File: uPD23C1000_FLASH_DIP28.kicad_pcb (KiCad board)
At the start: 2 copper layers, 16.6 x 34.4 mm, 8 parts, among them J1 uPD23C1000, J2 Conn_1x2, J3 Conn_1x3, U1 29F010 TSOP-32 20mm, U2 29F010 sTSOP-32 14mm, U3 29F010 PLCC-32 7x9

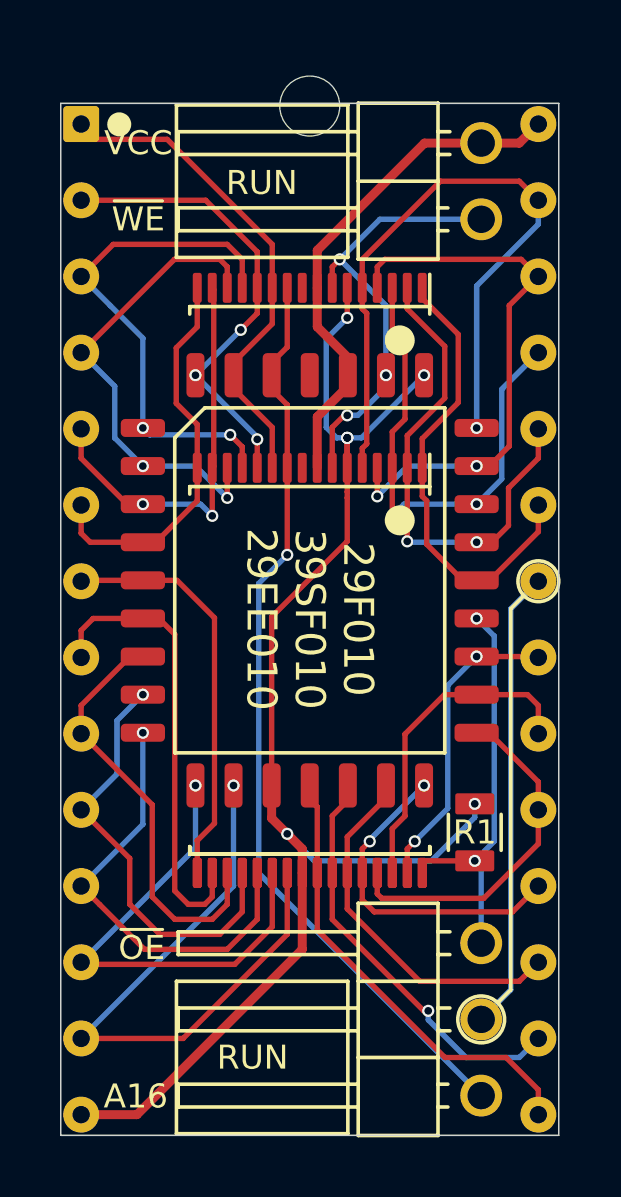
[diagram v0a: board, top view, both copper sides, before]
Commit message: minor touches
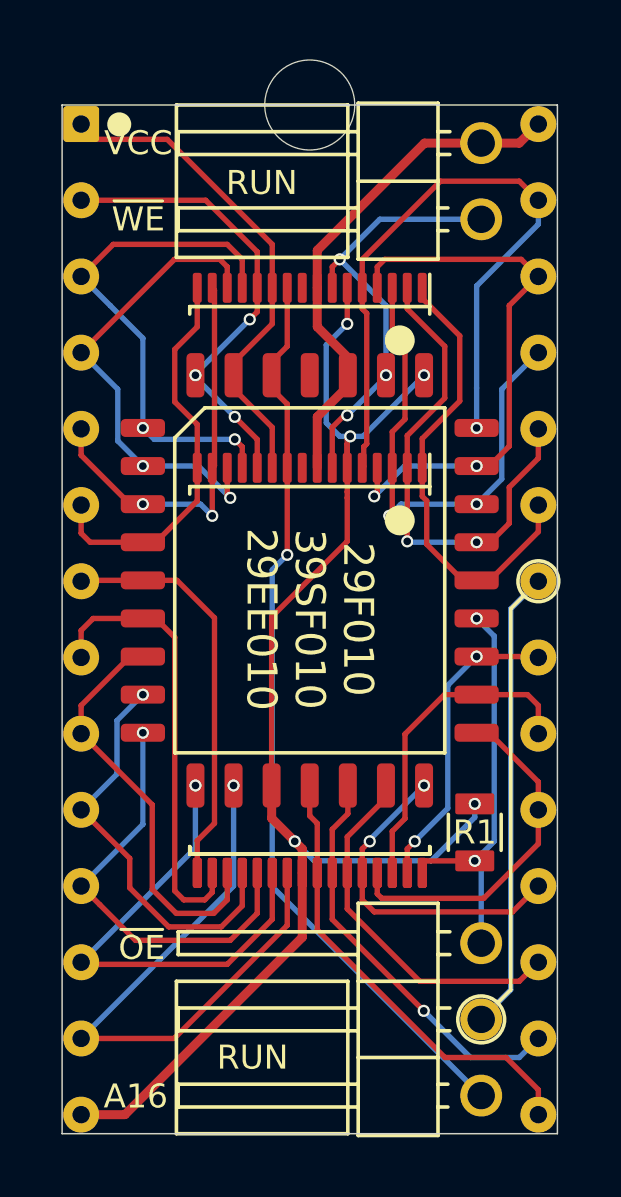
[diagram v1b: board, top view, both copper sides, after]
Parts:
- added REF**: NPTH_3mm, 000_LOCAL:NPTH_3mm, F.Cu at (150.0, 81.6)
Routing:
- net /A0: track 14.3 -> 13.7 mm
- net /GND: track 33.8 -> 33.3 mm
- net /A17: track 12.0 -> 11.8 mm, vias 4 -> 3
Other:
- board size 16.6 x 34.4 mm -> 16.5 x 34.3 mm
